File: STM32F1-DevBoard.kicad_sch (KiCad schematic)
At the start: 39 parts, among them J1 USB_C_Receptacle_USB2.0, SW1 SW_Push, SW2 SW_Push, U1 STM32F103C8T6, U2 AMS1117-3.3, U3 W25Q32JVSS

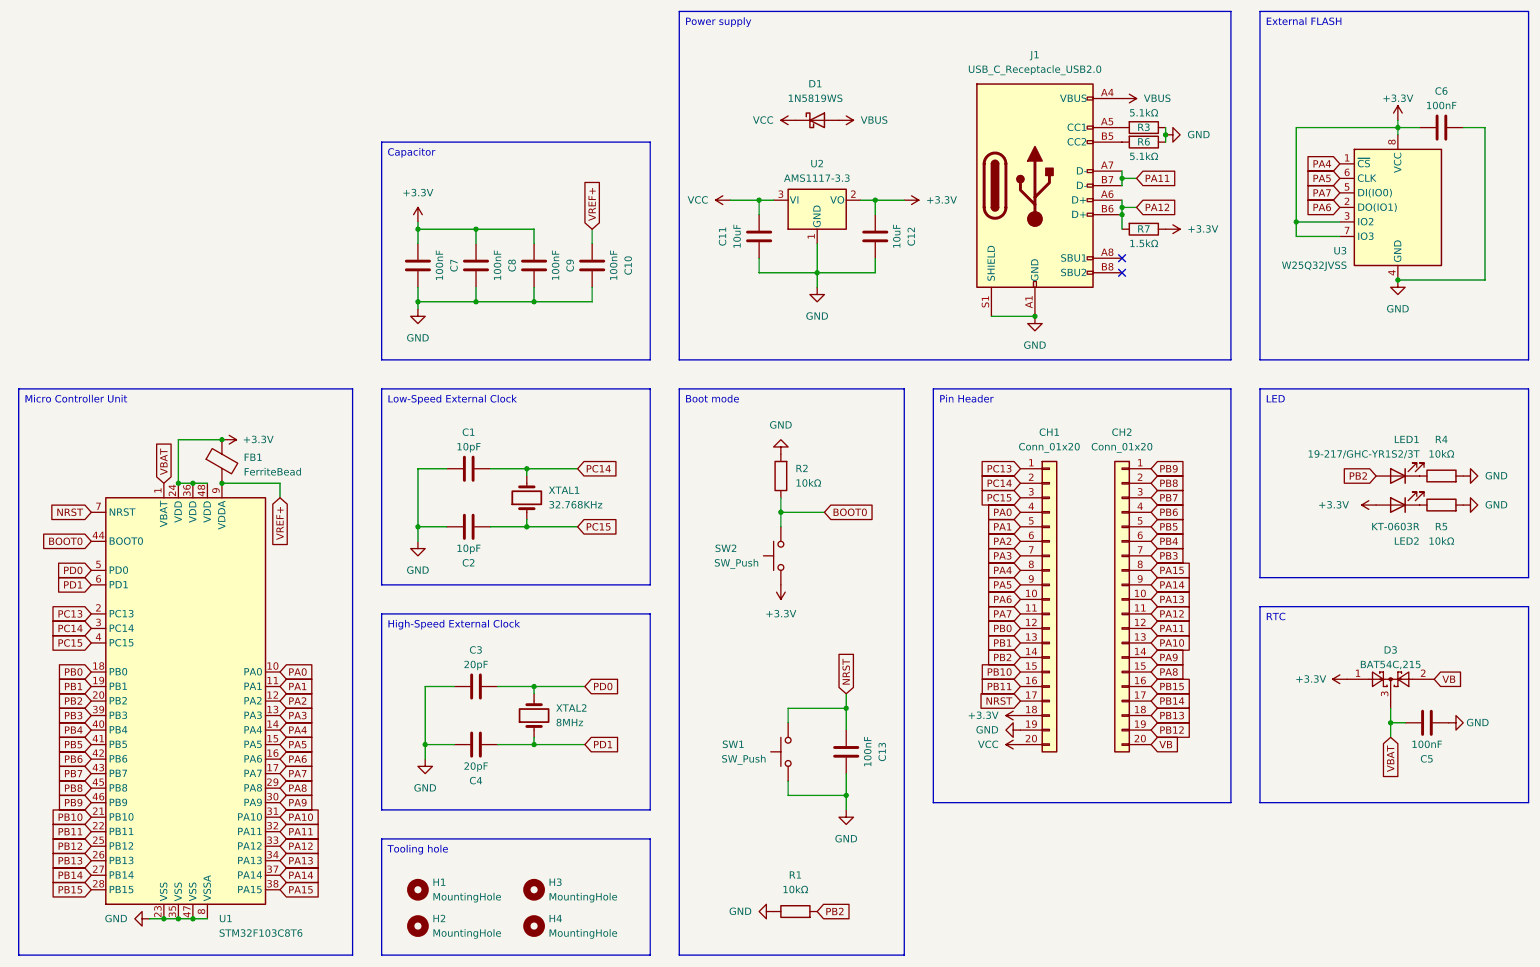
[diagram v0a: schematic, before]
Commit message: Add files via upload
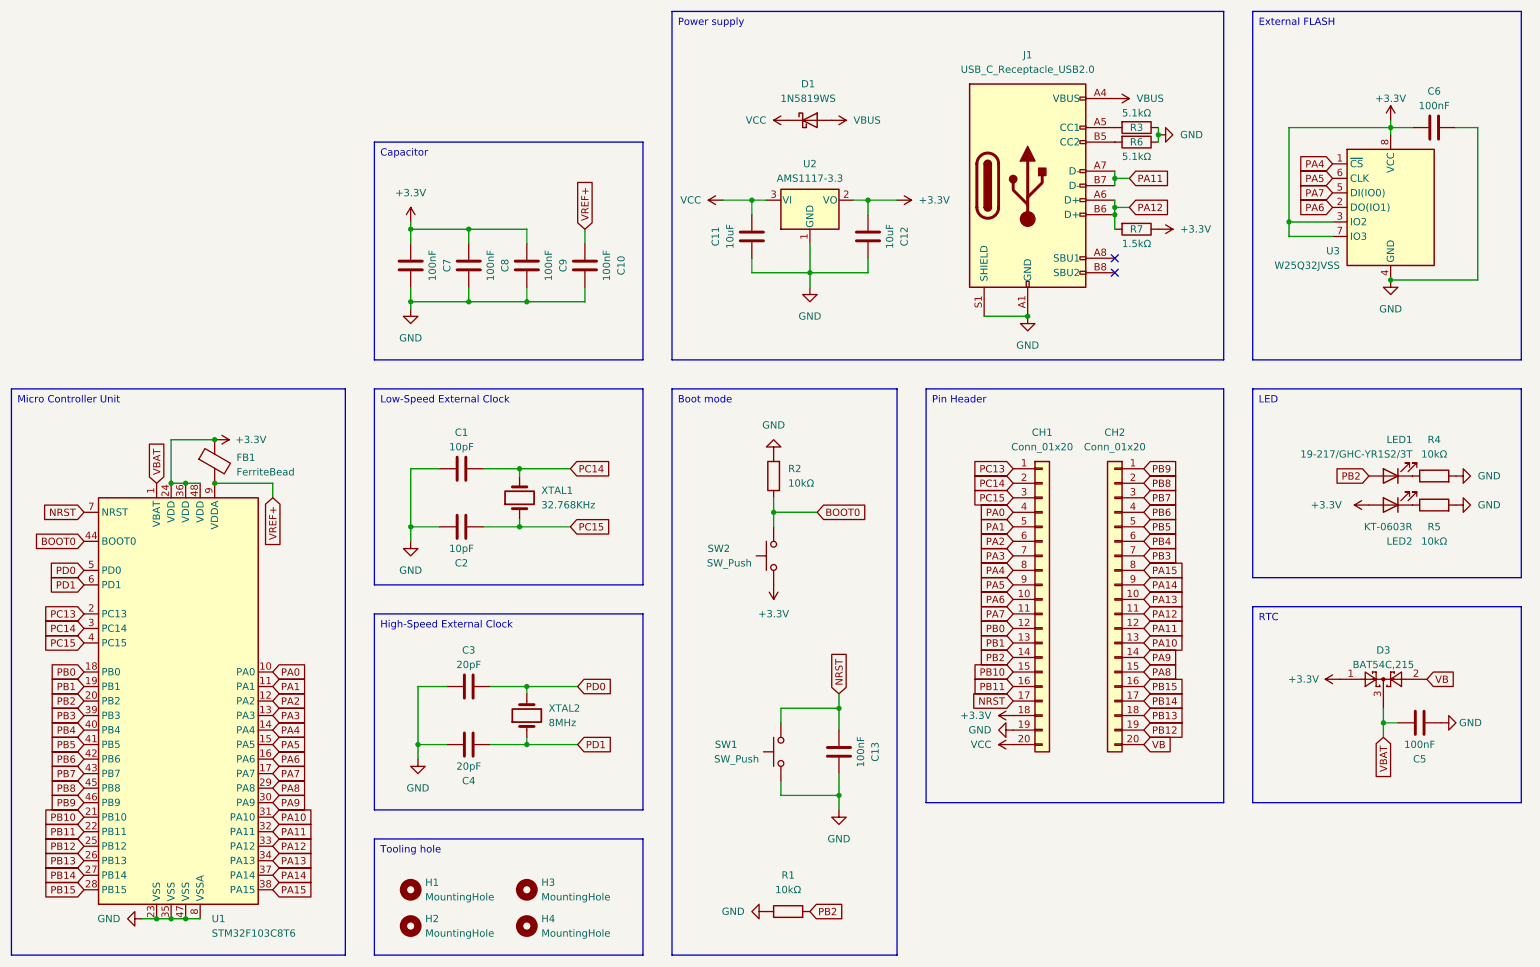
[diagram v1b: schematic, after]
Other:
- moved on the sheet: C1, C10, C11, C12, C13, C2, C3, C4, C5, C6, C7, C8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
